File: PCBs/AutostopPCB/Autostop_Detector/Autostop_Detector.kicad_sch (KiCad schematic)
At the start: 13 parts, among them J5 DSUB9 to backplane, P1 282837-2, U1 ESP32-S3-DevKitC, U2 SN65HVD230

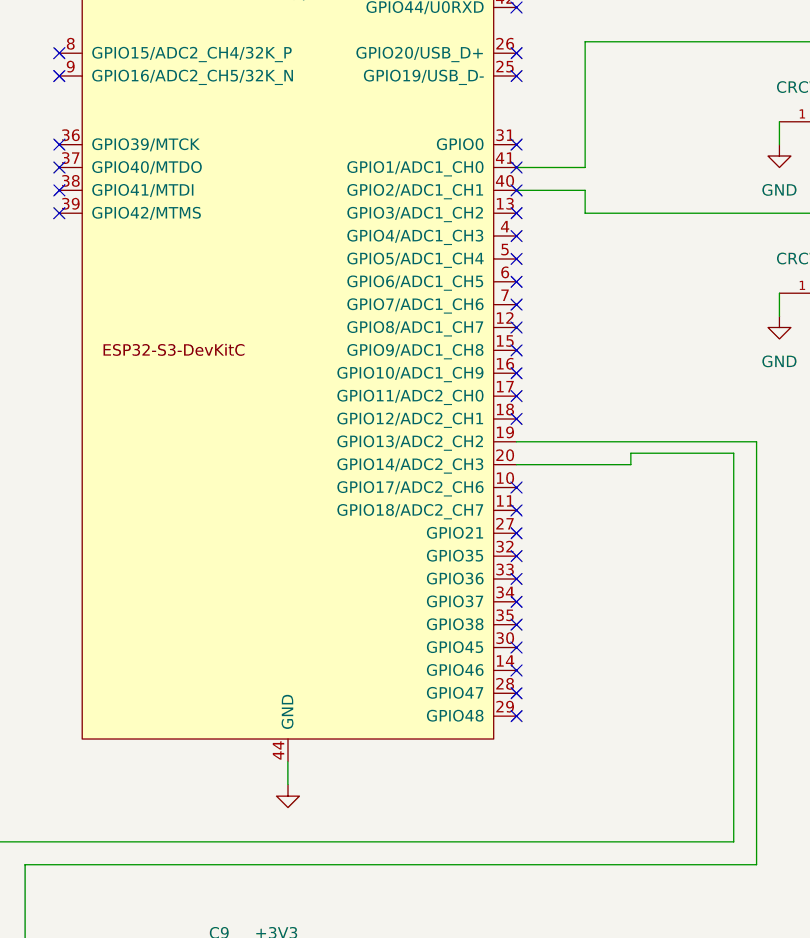
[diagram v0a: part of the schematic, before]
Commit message: Reapply "added driver controls v2"
This reverts commit d70487c3c1110107dce6cdfc2b36a156bfb5c696.
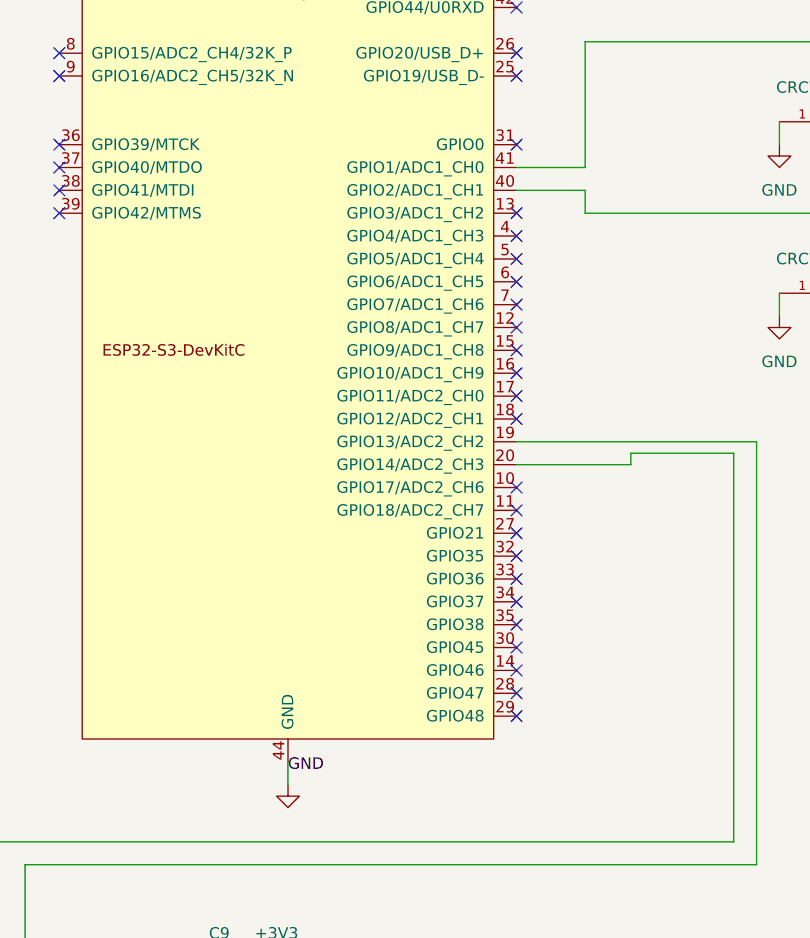
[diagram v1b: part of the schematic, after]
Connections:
- no-connect marks 41 -> 39
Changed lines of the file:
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@@
-	)
-	(no_connect
-		(at 76.2 63.5)
 	)
 	(no_connect
@@
 	(no_connect
 		(at 76.2 119.38)
-	)
-	(no_connect
-		(at 76.2 66.04)
 	)
 	(no_connect
@@
 		(effects
 			(font
+				(size 1.27 1.27)
+			)
+			(justify left bottom)
+		)
+	)
+	(label "GND"
+		(at 50.8 130.81 0)
+		(effects
+			(font

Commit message: Revert "added driver controls v2"
This reverts commit c73e8f860f70517a898f0b3e351800c05ab551df.
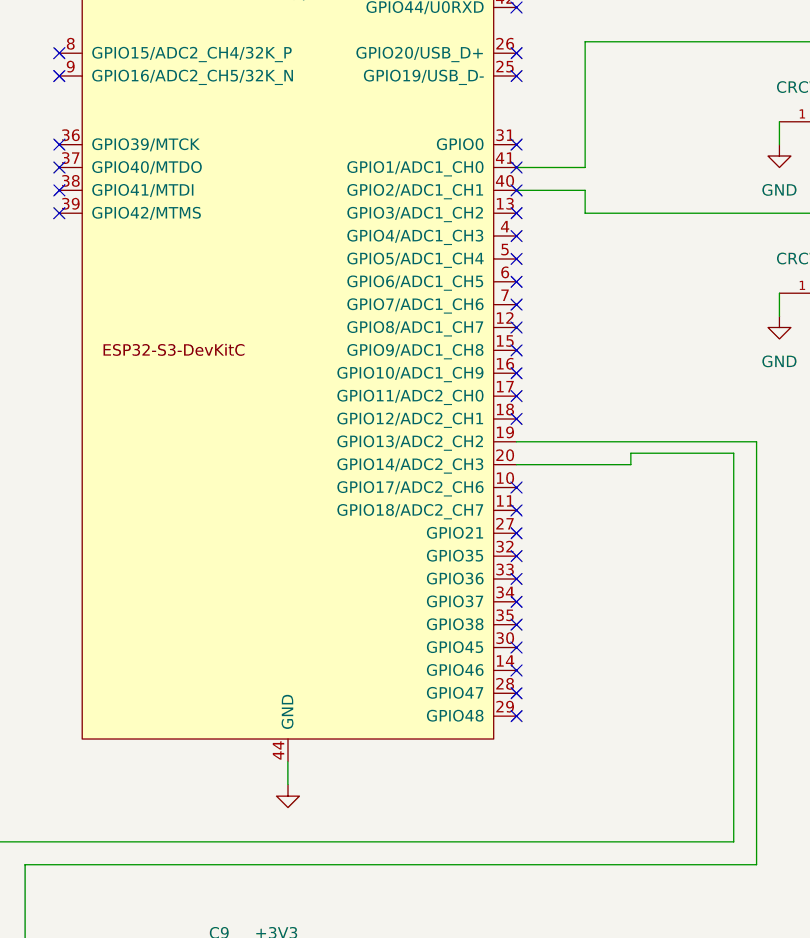
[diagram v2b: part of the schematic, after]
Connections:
- no-connect marks 39 -> 41
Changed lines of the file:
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@@
+	)
+	(no_connect
+		(at 76.2 63.5)
 	)
 	(no_connect
@@
 	(no_connect
 		(at 76.2 119.38)
+	)
+	(no_connect
+		(at 76.2 66.04)
 	)
 	(no_connect
@@
 		(effects
 			(font
-				(size 1.27 1.27)
-			)
-			(justify left bottom)
-		)
-	)
-	(label "GND"
-		(at 50.8 130.81 0)
-		(effects
-			(font
